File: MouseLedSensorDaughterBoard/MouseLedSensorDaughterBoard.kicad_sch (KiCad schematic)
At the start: 4 parts, among them J2 Conn_01x04

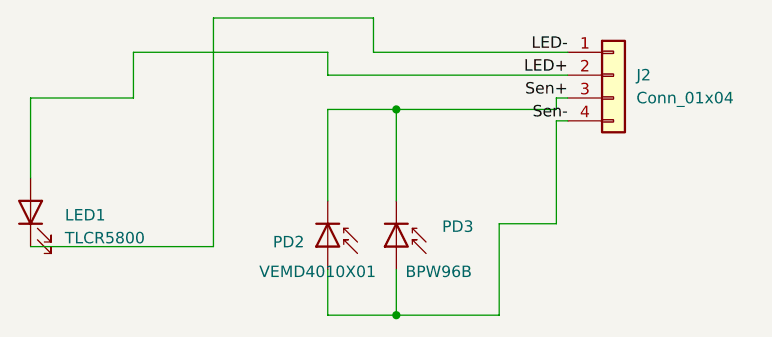
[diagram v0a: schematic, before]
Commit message: Sort of ready for JLCPCB
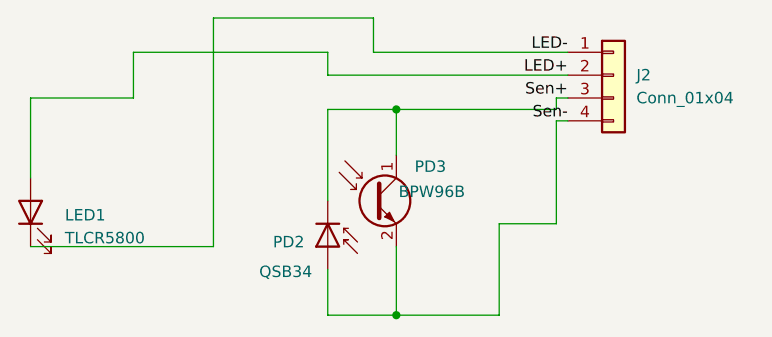
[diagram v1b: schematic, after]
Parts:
- PD2: value VEMD4010X01 -> QSB34; footprint Diode_SMD:D_0805_2012Metric_Pad1.15x1.40mm_HandSolder -> PBFootPrintLibrary:PLCC_2L_Handsoldering
- PD3: footprint LED_THT:LED_D5.0mm -> LED_THT:LED_D5.0mm_Clear; symbol Device:D_Photo -> Sensor_Optical:BPW40
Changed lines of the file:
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@@
 	(wire
 		(pts
-			(xy 160.02 102.87) (xy 160.02 107.95)
+			(xy 160.02 100.33) (xy 160.02 107.95)
 		)
 		(stroke
@@
 	(wire
 		(pts
-			(xy 160.02 85.09) (xy 160.02 95.25)
+			(xy 160.02 85.09) (xy 160.02 90.17)
 		)
 		(stroke
@@
 	(label "Sen+"
 		(at 179.07 83.82 180)
-		(fields_autoplaced yes)
 		(effects
 			(font
@@
 	(label "LED+"
 		(at 179.07 81.28 180)
-		(fields_autoplaced yes)
 		(effects
 			(font
@@
 	(label "Sen-"
 		(at 179.07 86.36 180)
-		(fields_autoplaced yes)
 		(effects
 			(font
@@
 	(label "LED-"
 		(at 179.07 78.74 180)
-		(fields_autoplaced yes)
 		(effects
 			(font
@@
 			)
 		)
-		(property "Value" "VEMD4010X01"
+		(property "Value" "QSB34"
 			(at 144.78 103.124 90)
 			(effects
@@
 			)
 		)
-		(property "Footprint" "Diode_SMD:D_0805_2012Metric_Pad1.15x1.40mm_HandSolder"
+		(property "Footprint" "PBFootPrintLibrary:PLCC_2L_Handsoldering"
 			(at 152.4 99.06 0)
 			(effects
@@
 	)
 	(symbol
-		(lib_id "Device:D_Photo")
-		(at 160.02 100.33 270)
+		(lib_id "Sensor_Optical:BPW40")
+		(at 157.48 95.25 0)
 		(unit 1)
 		(exclude_from_sim no)
@@
 		(dnp no)
 		(property "Reference" "PD3"
-			(at 165.1 98.1074 90)
+			(at 162.052 91.44 0)
 			(effects
 				(font
@@
 		)
 		(property "Value" "BPW96B"
-			(at 161.036 103.124 90)
-			(effects
-				(font
-					(size 1.27 1.27)
-				)
-				(justify left)
-			)
-		)
-		(property "Footprint" "LED_THT:LED_D5.0mm"
-			(at 160.02 99.06 0)
-			(effects
-				(font
-					(size 1.27 1.27)
-				)
-				(hide yes)
-			)
-		)
-		(property "Datasheet" "~"
-			(at 160.02 99.06 0)
-			(effects
-				(font
-					(size 1.27 1.27)
-				)
-				(hide yes)
-			)
-		)
-		(property "Description" "Photodiode"
-			(at 160.02 100.33 0)
-			(effects
-				(font
+			(at 160.274 94.234 0)
+			(effects
+				(font
+					(size 1.27 1.27)
+				)
+				(justify left)
+			)
+		)
+		(property "Footprint" "LED_THT:LED_D5.0mm_Clear"
+			(at 169.672 98.806 0)
+			(effects
+				(font
+					(size 1.27 1.27)
+				)
+				(hide yes)
+			)
+		)
+		(property "Datasheet" "https://www.rcscomponents.kiev.ua/datasheets/bpw40.pdf"
+			(at 157.48 95.25 0)
+			(effects
+				(font
+					(size 1.27 1.27)
+				)
+				(hide yes)
+			)
+		)
+		(property "Description" "Phototransistor NPN"
+			(at 157.48 95.25 0)
+			(effects
+				(font
